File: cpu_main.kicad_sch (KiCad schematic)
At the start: 18 parts, among them Q1 9018G, U1 Z80, U10 2764, U2 74LS244, U3 74LS257, U4 74LS257, U5 74LS00, U6 27128, U7 27128/27256, U8 GA1, U9 74LS273

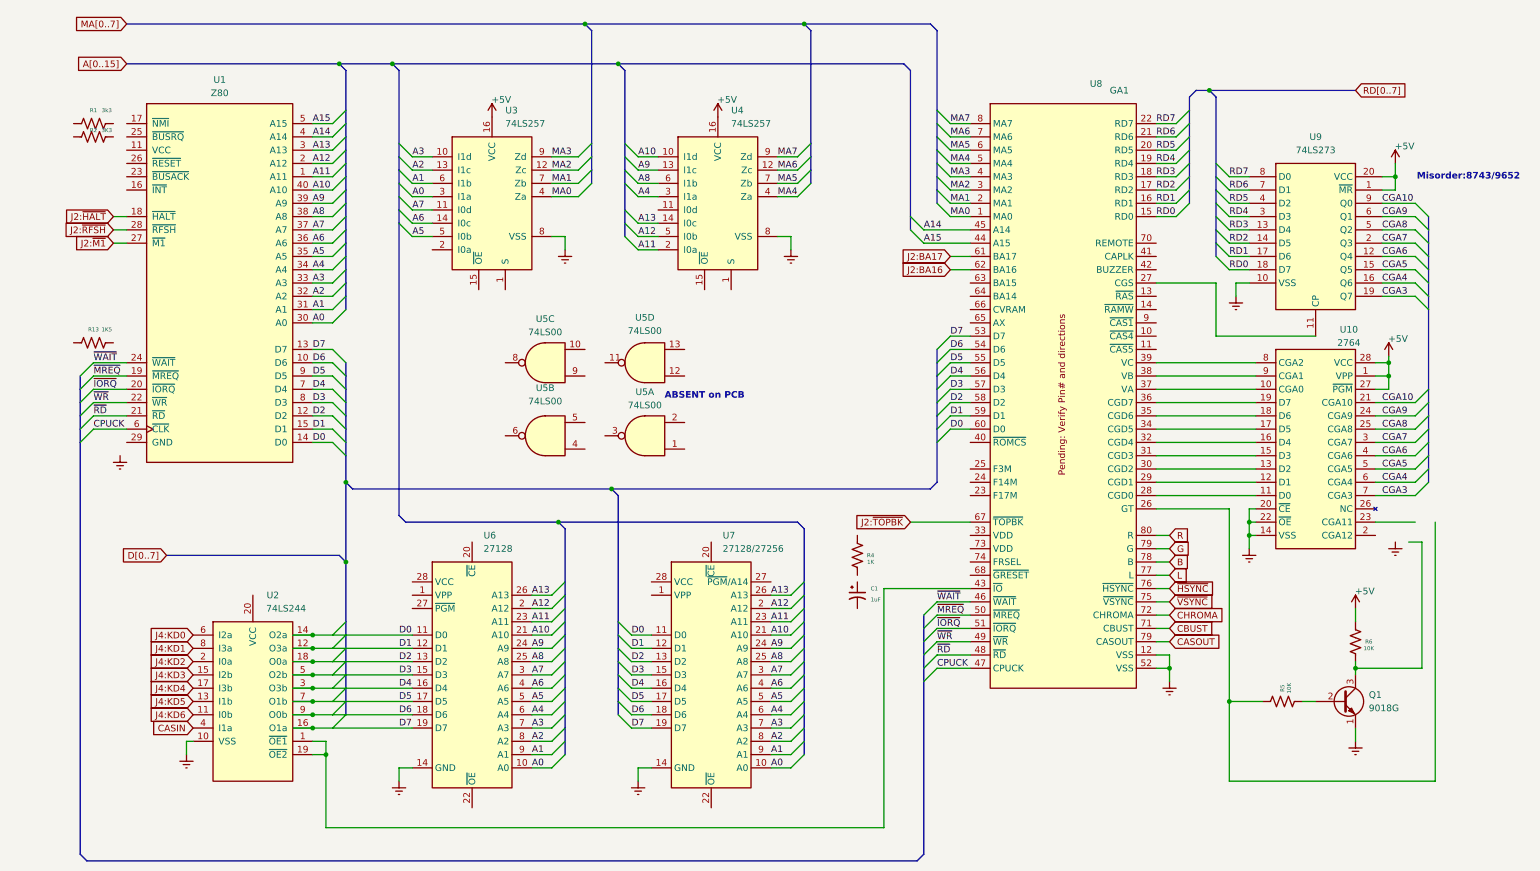
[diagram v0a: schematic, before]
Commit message: End of vacation
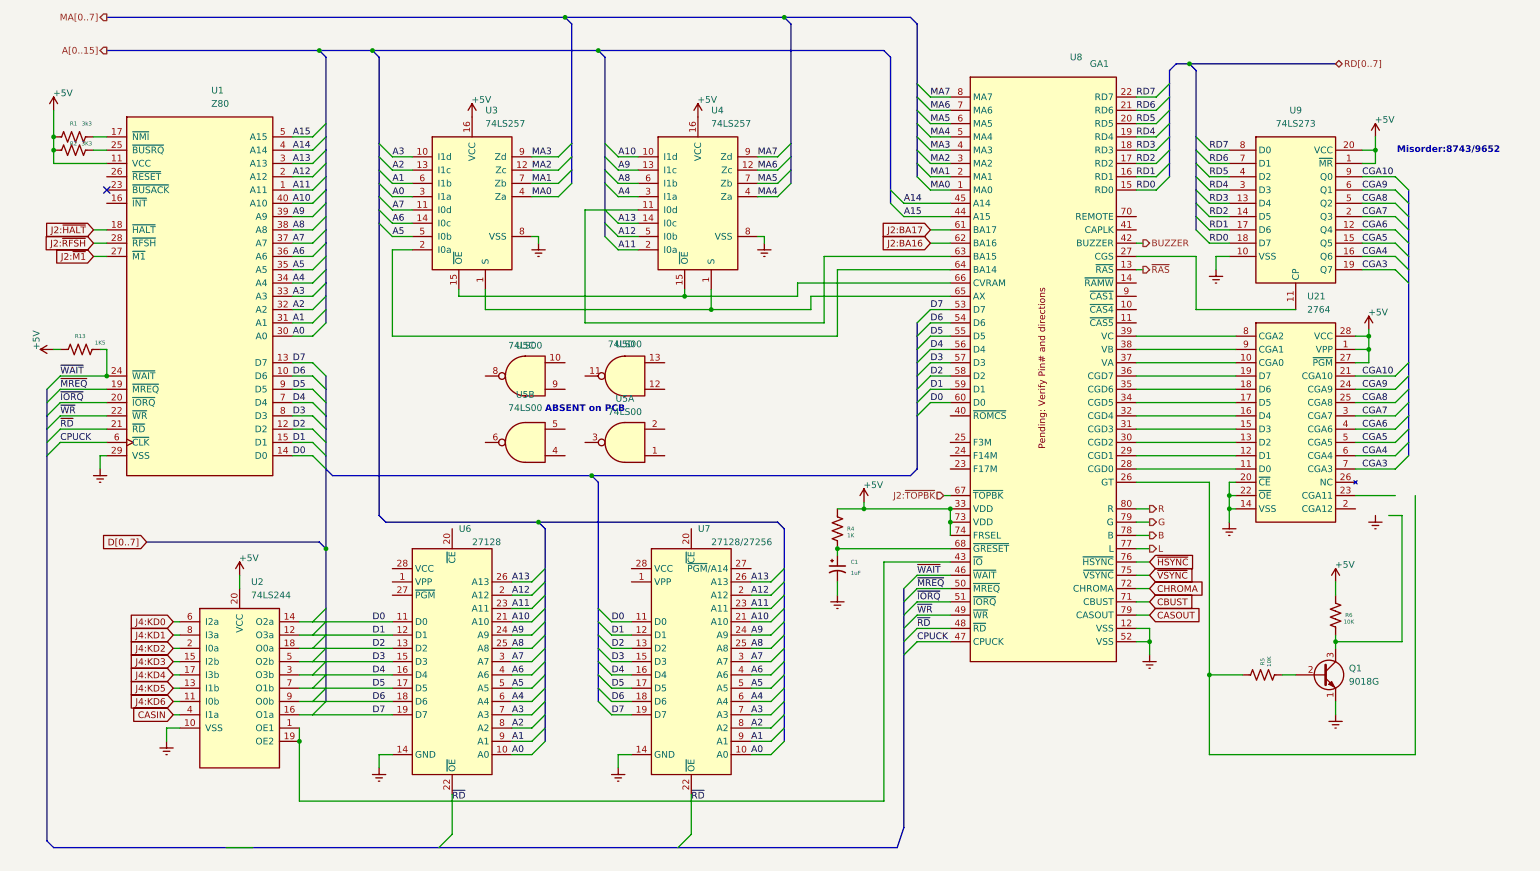
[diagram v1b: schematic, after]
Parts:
- removed U1: Z80, symbol Laser500:Z80
- removed U10: 2764, Package_DIP:DIP-28_W15.24mm, symbol Laser500:2764
- removed U2: 74LS244, symbol Laser500:74LS244
- added U1: Z80, symbol CPU:Z80CPU
- added U2: 74LS244, symbol 74xx:74LS244
- added U21: 2764, Package_DIP:DIP-28_W15.24mm, symbol Memory_EPROM:2764
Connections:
- net +5V: now also R1.2, R13.2, R2.2, R4.2, U8.33 (VDD), U8.73 (VDD), U8.74 (FRSEL), U1.11 (VCC), U2.20 (VCC), U21.1 (VPP), U21.27 (~{PGM}), U21.28 (VCC)
- net A0: now also U1.30 (A0)
- net A1: now also U1.31 (A1)
- net A10: now also U1.40 (A10)
- net A11: now also U1.1 (A11)
- net A12: now also U1.2 (A12)
- net A13: now also U1.3 (A13)
- net A14: now also U1.4 (A14)
- net A15: now also U1.5 (A15)
- net A2: now also U1.32 (A2)
- net A3: now also U1.33 (A3)
- net A4: now also U1.34 (A4)
- net A5: now also U1.35 (A5)
- net A6: now also U1.36 (A6)
- net A7: now also U1.37 (A7)
- net A8: now also U1.38 (A8)
- net A9: now also U1.39 (A9)
- net CASIN: now also U2.4 (I1a)
- net CGA10: now also U21.21 (CGA10)
- net CGA3: now also U21.7 (CGA3)
- net CGA4: now also U21.6 (CGA4)
- net CGA5: now also U21.5 (CGA5)
- net CGA6: now also U21.4 (CGA6)
- net CGA7: now also U21.3 (CGA7)
- net CGA8: now also U21.25 (CGA8)
- net CGA9: now also U21.24 (CGA9)
- net CPUCK: now also U1.6 (~{CLK})
- net D0: now also U1.14 (D0), U2.14 (O2a)
- net D1: now also U1.15 (D1), U2.12 (O3a)
- net D2: now also U1.12 (D2), U2.18 (O0a)
- net D3: now also U1.8 (D3), U2.5 (O2b)
- net D4: now also U1.7 (D4), U2.3 (O3b)
- net D5: now also U1.9 (D5), U2.7 (O1b)
- net D6: now also U1.10 (D6), U2.9 (O0b)
- net D7: now also U1.13 (D7), U2.16 (O1a)
- net J2:~{HALT}: now also U1.18 (~{HALT})
- net J2:~{M1}: now also U1.27 (~{M1})
- net J2:~{RFSH}: now also U1.28 (~{RFSH})
- net J4:KD0: now also U2.6 (I2a)
- net J4:KD1: now also U2.8 (I3a)
- net J4:KD2: now also U2.2 (I0a)
- net J4:KD3: now also U2.15 (I2b)
- net J4:KD4: now also U2.17 (I3b)
- net J4:KD5: now also U2.13 (I1b)
- net J4:KD6: now also U2.11 (I0b)
- net ~{IORQ}: now also U1.20 (~{IORQ})
- net ~{MREQ}: now also U1.19 (~{MREQ})
- net ~{RD}: now also U6.22 (~{OE}), U7.22 (~{OE}), U8.43 (~{IO}), U1.21 (~{RD}), U2.1 (OE1), U2.19 (OE2)
- net ~{WAIT}: now also R13.1, U1.24 (~{WAIT})
- net ~{WR}: now also U1.22 (~{WR})
- net at U3.1 (S): now also U4.1 (S), U8.65 (AX)
- net at U3.15 (~{OE}): now also U4.15 (~{OE}), U8.66 (CVRAM)
- net at U3.2 (I0a): now also U8.64 (BA14)
- net at C1.1: now also R4.1, U8.68 (~{GRESET})
- net at R1.1: now also U1.17 (~{NMI})
- net at U8.37 (VA): now also U21.10 (CGA0)
- net at U8.28 (CGD0): now also U21.11 (D0)
- net at U8.29 (CGD1): now also U21.12 (D1)
- net at U8.30 (CGD2): now also U21.13 (D2)
- net at U8.31 (CGD3): now also U21.15 (D3)
- net at U8.32 (CGD4): now also U21.16 (D4)
- net at U8.34 (CGD5): now also U21.17 (D5)
- net at U8.35 (CGD6): now also U21.18 (D6)
- net at U8.36 (CGD7): now also U21.19 (D7)
- net at U8.39 (VC): now also U21.8 (CGA2)
- net at U8.38 (VB): now also U21.9 (CGA1)
- net at U4.11 (I0d): now also U8.63 (BA15)
- net at R2.1: now also U1.25 (~{BUSRQ})
- net ~{RAS}: now reaches U8.13 (~{RAS})
- net BUZZER: now reaches U8.42 (BUZZER)
- new net: U21.14 (VSS), U21.20 (~{CE}), U21.22 (~{OE})
- no-connect marks 0 -> 1
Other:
- moved on the sheet: C1, Q1, R1, R13, R2, R4, R5, R6, U3, U4, U5A, U5B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
